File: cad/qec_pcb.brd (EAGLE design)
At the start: 53.6 x 35.6 mm, 6 parts, among them K1 68611114122

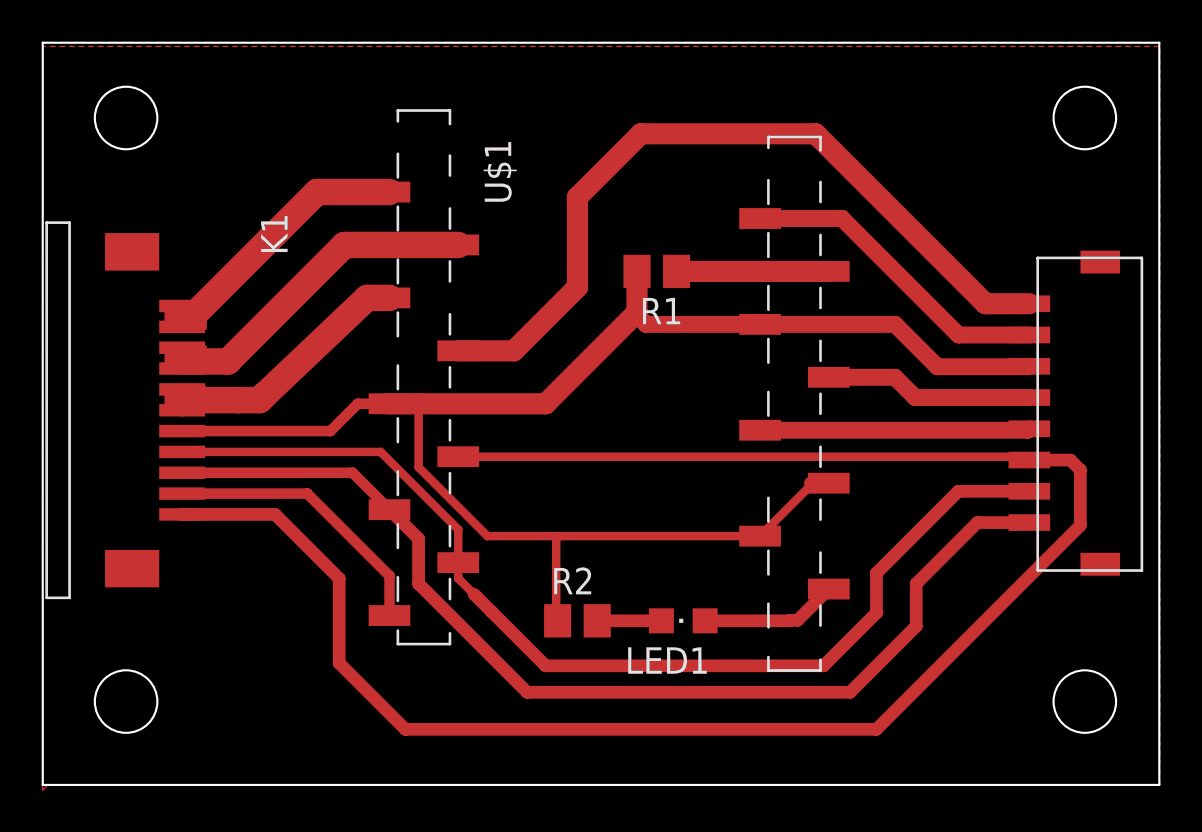
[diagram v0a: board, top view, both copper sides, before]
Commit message: update pcb for production
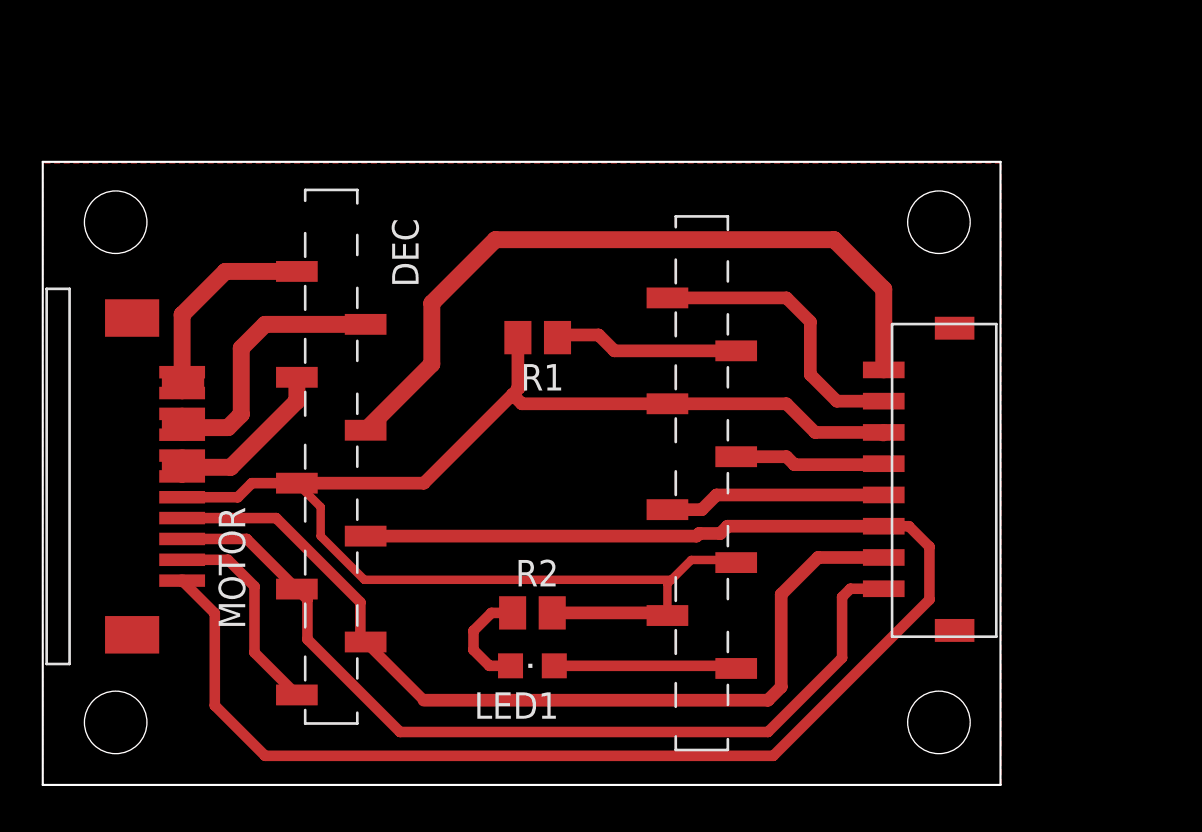
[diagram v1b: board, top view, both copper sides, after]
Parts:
- removed K1: 68611114122, dedo:68611114122
- removed U$1: 1-Q-EC1-Q-EC-SMD, dedo:1-Q-EC-SMD
- added DEC: 1-Q-EC1-Q-EC-SMD, dedo:1-Q-EC-SMD
- added MOTOR: 68611114122, dedo:68611114122
- moved CTRL 7.67 mm to (43.1, 15.1)
- moved LED1 7.55 mm to (23.5, 5.71)
- moved R1 6.54 mm to (23.7, 21.5)
- moved R2 2.19 mm to (23.5, 8.26), turned to 180 degrees
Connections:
- removed net N$16: K1.2, U$1.9
- new net H3: DEC.9, MOTOR.2
- net +24V: now also DEC.4; no longer U$1.4
- net DIR: now also DEC.14; no longer U$1.14
- net EN: now also DEC.13; no longer U$1.13
- net GND: now also DEC.11, DEC.12, DEC.15, DEC.5, MOTOR.5; no longer K1.5, U$1.11, U$1.12, U$1.15, U$1.5
- net H1: now also DEC.7, MOTOR.3; no longer K1.3, U$1.7
- net H2: now also DEC.8, MOTOR.4; no longer K1.4, U$1.8
- net N$11: now also DEC.2, MOTOR.8, MOTOR.9; no longer K1.8, K1.9, U$1.2
- net N$12: now also DEC.3, MOTOR.6, MOTOR.7; no longer K1.6, K1.7, U$1.3
- net N$2: now also DEC.10; no longer U$1.10
- net N$5: now also DEC.1, MOTOR.10, MOTOR.11; no longer K1.10, K1.11, U$1.1
- net N$6: now also DEC.16; no longer U$1.16
- net SVS: now also DEC.17; no longer U$1.17
- net V+: now also DEC.6, MOTOR.1; no longer K1.1, U$1.6
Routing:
- net N$16: track 13.5 -> 0.00 mm
- net V+: track 87.0 -> 75.3 mm
- net H3: track 0.00 -> 10.1 mm
- net N$12: track 18.7 -> 9.14 mm
- net N$11: track 22.2 -> 13.7 mm
- net H1: track 51.6 -> 43.2 mm
- net H2: track 52.0 -> 43.7 mm
- net GND: track 78.2 -> 73.2 mm
- net N$5: track 15.1 -> 10.1 mm
- net DIR: track 10.9 -> 7.44 mm
- net +24V: track 37.6 -> 35.2 mm
- net N$2: track 6.56 -> 8.78 mm
- net N$1: track 3.08 -> 5.24 mm
- net EN: track 12.9 -> 10.9 mm
- net N$6: track 7.30 -> 8.94 mm
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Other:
- board size 53.6 x 35.6 mm -> 46 x 29.9 mm
